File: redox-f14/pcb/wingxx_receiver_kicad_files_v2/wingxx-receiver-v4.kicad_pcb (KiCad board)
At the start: 2 copper layers, 78.7 x 90.2 mm, 61 parts, among them K1 KEYSW-redox_rev1-rescue, K11 KEYSW-redox_rev1-rescue, K12 KEYSW-redox_rev1-rescue, K13 KEYSW-redox_rev1-rescue, K14 KEYSW-redox_rev1-rescue, K2 KEYSW-redox_rev1-rescue, K21 KEYSW-redox_rev1-rescue, K22 KEYSW-redox_rev1-rescue, K23 KEYSW-redox_rev1-rescue, K24 KEYSW-redox_rev1-rescue, K3 KEYSW-redox_rev1-rescue, K31 KEYSW-redox_rev1-rescue, K32 KEYSW-redox_rev1-rescue, K33 KEYSW-redox_rev1-rescue, K34 KEYSW-redox_rev1-rescue, K4 KEYSW-redox_rev1-rescue, U1 ATmega32U4-AU, X1 Crystal_GND24

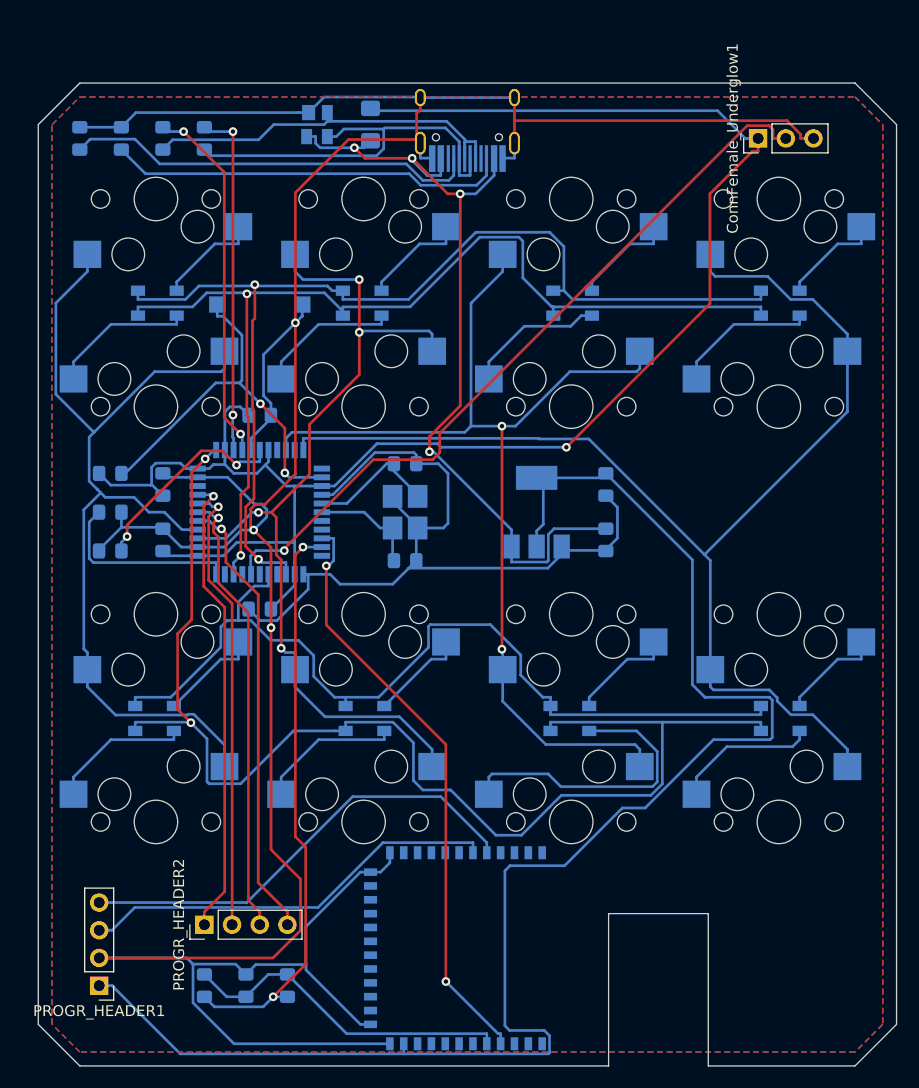
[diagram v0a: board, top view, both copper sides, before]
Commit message: new receiver
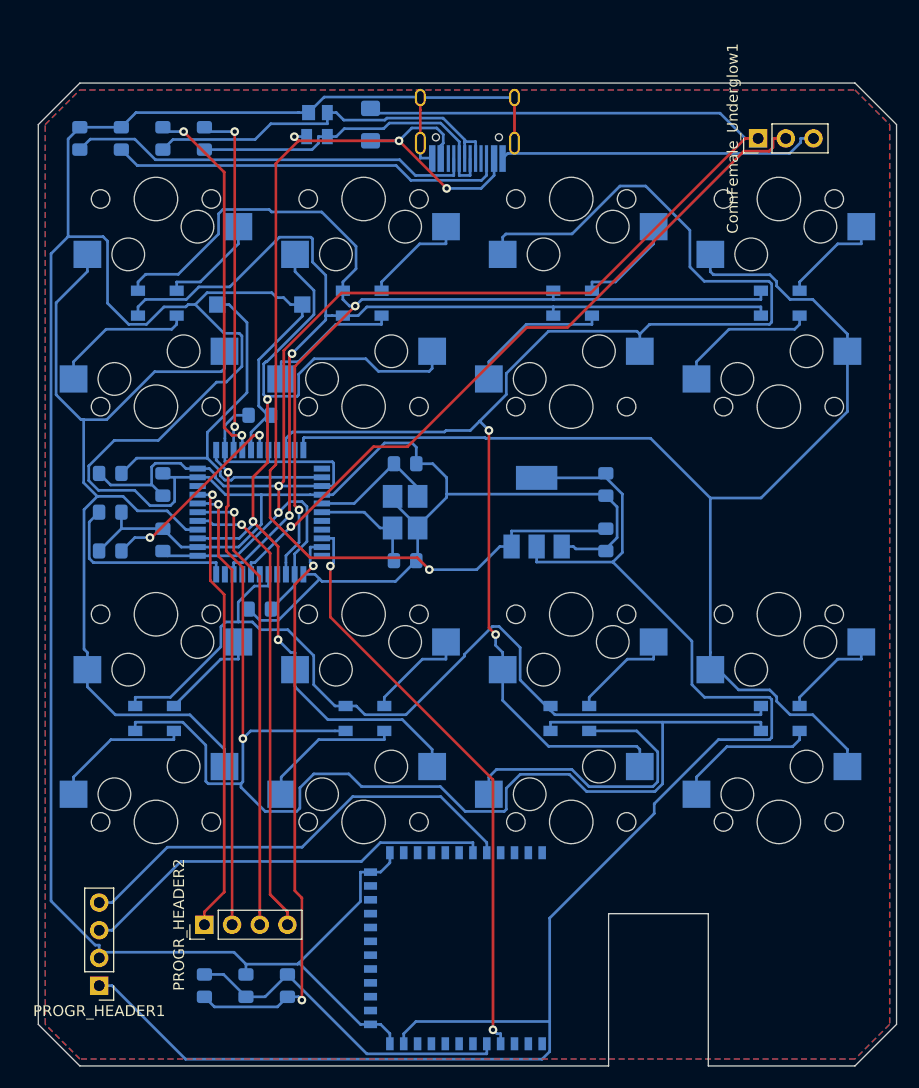
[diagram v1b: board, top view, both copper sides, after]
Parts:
- D1, D11, D12, D13, D14, D2, D21, D22, D23, D24, D3, D31, D32, D33, D34, D4: footprint pcb:D3_SMD_Back -> pcb:D3_SMD_Front; moved to B.Cu
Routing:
- net col2: track 96.0 -> 132.9 mm
- net GND: track 375.6 -> 402.5 mm, vias 3 -> 0
- net VCC: track 78.3 -> 104.0 mm
- net +5V: track 156.7 -> 175.2 mm, vias 1 -> 2
- net row3: track 118.6 -> 130.3 mm
- net +3.3V: track 141.8 -> 148.8 mm
- net Net-(D6-Pad3): track 37.4 -> 31.1 mm
- net col1: track 82.6 -> 87.2 mm, vias 4 -> 3
- net RGB_DATA: track 69.3 -> 66.7 mm
- net row1: track 95.3 -> 96.6 mm
- net POF5: track 41.3 -> 42.6 mm
- net Net-(R5-Pad2): track 36.4 -> 37.5 mm, vias 2 -> 0
- net Net-(C3-Pad1): track 19.3 -> 18.4 mm
- net POF4: track 41.4 -> 42.2 mm
- net row0: track 98.7 -> 99.4 mm
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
